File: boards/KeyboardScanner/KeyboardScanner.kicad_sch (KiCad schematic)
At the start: 20 parts, among them J1 Keyboard1, J2 Keyboard1, J3 Encoder, J4 Select, U11 TBD62783A, U8 4069

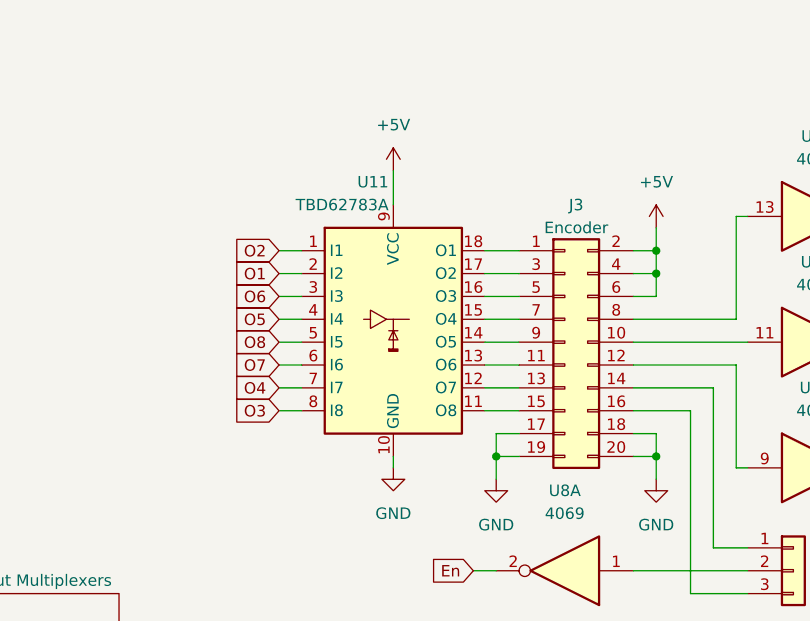
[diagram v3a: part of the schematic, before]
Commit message: Revert "Replaced inverting with non-inverting output buffer in KeyboardScanner to fix disabled open collector output"
This reverts commit 6ddf25a0a7a31b9f16f3f110cd3b7ae66d122c97.
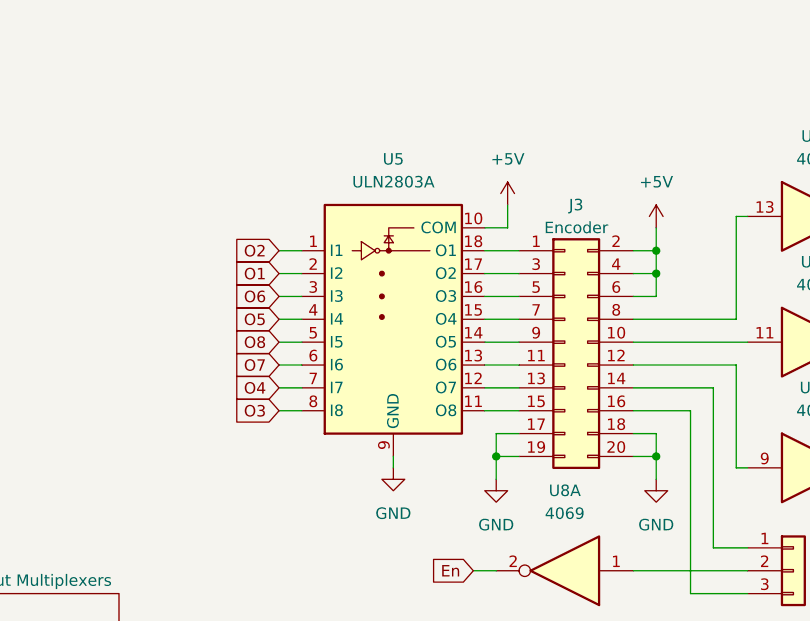
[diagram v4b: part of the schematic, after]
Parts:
- removed U11: TBD62783A, Package_DIP:DIP-18_W7.62mm, symbol Transistor_Array:TBD62783A
- added U5: ULN2803A, Package_DIP:DIP-18_W7.62mm, symbol Transistor_Array:ULN2803A
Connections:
- net +5V: now also U5.10 (COM)
- net GND: now also U5.9 (GND)
- net O1: now also U5.2 (I2)
- net O2: now also U5.1 (I1)
- net O3: now also U5.8 (I8)
- net O4: now also U5.7 (I7)
- net O5: now also U5.4 (I4)
- net O6: now also U5.3 (I3)
- net O7: now also U5.6 (I6)
- net O8: now also U5.5 (I5)
- net at J3.1 (Pin_1): now also U5.18 (O1)
- net at J3.11 (Pin_11): now also U5.13 (O6)
- net at J3.13 (Pin_13): now also U5.12 (O7)
- net at J3.15 (Pin_15): now also U5.11 (O8)
- net at J3.3 (Pin_3): now also U5.17 (O2)
- net at J3.5 (Pin_5): now also U5.16 (O3)
- net at J3.7 (Pin_7): now also U5.15 (O4)
- net at J3.9 (Pin_9): now also U5.14 (O5)
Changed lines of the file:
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@@
 	(wire
 		(pts
+			(xy 194.31 48.26) (xy 191.77 48.26)
+		)
+		(stroke
+			(width 0)
+			(type default)
+		)
+	)
+	(wire
+		(pts
 			(xy 208.28 86.36) (xy 220.98 86.36)
 		)
@@
 	(wire
 		(pts
+			(xy 194.31 45.72) (xy 194.31 48.26)
+		)
+		(stroke
+			(width 0)
+			(type default)
+		)
+	)
+	(wire
+		(pts
 			(xy 58.42 90.17) (xy 58.42 88.9)
 		)
@@
 	(wire
 		(pts
-			(xy 181.61 41.91) (xy 181.61 45.72)
-		)
-		(stroke
-			(width 0)
-			(type default)
-		)
-	)
-	(wire
-		(pts
 			(xy 45.72 76.2) (xy 63.5 76.2)
 		)
@@
 	(symbol
 		(lib_id "power:+5V")
-		(at 181.61 41.91 0)
+		(at 194.31 45.72 0)
 		(unit 1)
 		(exclude_from_sim no)
@@
 		(fields_autoplaced yes)
 		(property "Reference" "#PWR010"
-			(at 181.61 45.72 0)
+			(at 194.31 49.53 0)
 			(effects
 				(font
@@
 		)
 		(property "Value" "+5V"
-			(at 181.61 36.83 0)
+			(at 194.31 40.64 0)
 			(effects
 				(font
@@
 		)
 		(property "Footprint" ""
-			(at 181.61 41.91 0)
+			(at 194.31 45.72 0)
 			(effects
 				(font
@@
 		)
 		(property "Datasheet" ""
-			(at 181.61 41.91 0)
+			(at 194.31 45.72 0)
 			(effects
 				(font
@@
 		)
 		(property "Description" "Power symbol creates a global label with name \"+5V\""
-			(at 181.61 41.91 0)
+			(at 194.31 45.72 0)
 			(effects
 				(font
@@
 	)
 	(symbol
-		(lib_id "Transistor_Array:TBD62783A")
-		(at 181.61 58.42 0)
+		(lib_id "Device:C_Polarized")
+		(at 194.31 125.73 0)
 		(unit 1)
 		(exclude_from_sim no)
@@
 		(on_board yes)
 		(dnp no)
-		(property "Reference" "U11"
-			(at 181.0894 43.18 0)
+		(fields_autoplaced yes)
+		(property "Reference" "C10"
+			(at 198.12 123.5709 0)
 			(effects
 				(font
 					(size 1.27 1.27)
 				)
-				(justify right)
+				(justify left)
 			)
 		)
-		(property "Value" "TBD62783A"
-			(at 181.0894 45.72 0)
+		(property "Value" "47uF"
+			(at 198.12 126.1109 0)
 			(effects
 				(font
 					(size 1.27 1.27)
 				)
-				(justify right)
+				(justify left)
 			)
 		)
-		(property "Footprint" "Package_DIP:DIP-18_W7.62mm"
-			(at 181.61 72.39 0)
+		(property "Footprint" "Capacitor_THT:CP_Radial_D6.3mm_P2.50mm"
+			(at 195.2752 129.54 0)
 			(effects
 				(font
@@
 			)
 		)
-		(property "Datasheet" "http://toshiba.semicon-storage.com/info/docget.jsp?did=30523&prodName=TBD62783APG"
-			(at 173.99 48.26 0)
+		(property "Datasheet" "~"
+			(at 194.31 125.73 0)
 			(effects
 				(font
@@
 			)
 		)
-		(property "Description" "8-Channel Source Type Transistor Array, TTL and CMOS compatible, 500mA, 50V, DIP-18/SOP-18/SSOP-18/SOIC-18W"
-			(at 181.61 58.42 0)
+		(property "Description" "Polarized capacitor"
+			(at 194.31 125.73 0)
 			(effects
 				(font
@@
 			)
 		)
-		(pin "1"
-		)
-		(pin "10"
-		)
-		(pin "11"
-		)
-		(pin "12"
-		)
-		(pin "13"
-		)
-		(pin "14"
-		)
-		(pin "15"
-		)
-		(pin "16"
-		)
-		(pin "17"
-		)
-		(pin "18"
-		)
 		(pin "2"
 		)
-		(pin "3"
-		)
-		(pin "4"
-		)
-		(pin "5"
-		)
-		(pin "6"
-		)
-		(pin "7"
-		)
-		(pin "8"
-		)
-		(pin "9"
+		(pin "1"
 		)
 		(instances
 			(project "KeyboardScanner"
 				(path "/cbea9b23-a5d5-4e12-8904-2e66ea6ed837"
-					(reference "U11")
+					(reference "C10")
 					(unit 1)
 				)
@@
 	)
 	(symbol
-		(lib_id "Device:C_Polarized")
-		(at 194.31 125.73 0)
+		(lib_id "4xxx:4069")
+		(at 200.66 86.36 180)
 		(unit 1)
 		(exclude_from_sim no)
@@
 		(dnp no)
 		(fields_autoplaced yes)
-		(property "Reference" "C10"
-			(at 198.12 123.5709 0)
+		(property "Reference" "U8"
+			(at 200.66 77.47 0)
 			(effects
 				(font
 					(size 1.27 1.27)
 				)
-				(justify left)
 			)
 		)
-		(property "Value" "47uF"
-			(at 198.12 126.1109 0)
+		(property "Value" "4069"
+			(at 200.66 80.01 0)
 			(effects
 				(font
 					(size 1.27 1.27)
 				)
-				(justify left)
 			)
 		)
-		(property "Footprint" "Capacitor_THT:CP_Radial_D6.3mm_P2.50mm"
-			(at 195.2752 129.54 0)
+		(property "Footprint" "Package_DIP:DIP-14_W7.62mm"
+			(at 200.66 86.36 0)
 			(effects
 				(font
@@
 			)
 		)
-		(property "Datasheet" "~"
-			(at 194.31 125.73 0)
+		(property "Datasheet" "http://www.intersil.com/content/dam/Intersil/documents/cd40/cd4069ubms.pdf"
+			(at 200.66 86.36 0)
 			(effects
 				(font
@@
 			)
 		)
-		(property "Description" "Polarized capacitor"
-			(at 194.31 125.73 0)
+		(property "Description" "Hex inverter"
+			(at 200.66 86.36 0)
 			(effects
 				(font
@@
 			)
 		)
+		(pin "1"
+		)
 		(pin "2"
 		)
-		(pin "1"
+		(pin "3"
+		)
+		(pin "4"
+		)
+		(pin "5"
+		)
+		(pin "6"
+		)
+		(pin "8"
+		)
+		(pin "9"
+		)
+		(pin "10"
+		)
+		(pin "11"
+		)
+		(pin "12"
+		)
+		(pin "13"
+		)
+		(pin "14"
+		)
+		(pin "7"
 		)
 		(instances
 			(project "KeyboardScanner"
 				(path "/cbea9b23-a5d5-4e12-8904-2e66ea6ed837"
-					(reference "C10")
+					(reference "U8")
 					(unit 1)
 				)
@@
 	)
 	(symbol
-		(lib_id "4xxx:4069")
-		(at 200.66 86.36 180)
+		(lib_id "Transistor_Array:ULN2803A")
+		(at 181.61 55.88 0)
 		(unit 1)
 		(exclude_from_sim no)
@@
 		(dnp no)
 		(fields_autoplaced yes)
-		(property "Reference" "U8"
-			(at 200.66 77.47 0)
+		(property "Reference" "U5"
+			(at 181.61 40.64 0)
 			(effects
 				(font
@@
 			)
 		)
-		(property "Value" "4069"
-			(at 200.66 80.01 0)
+		(property "Value" "ULN2803A"
+			(at 181.61 43.18 0)
 			(effects
 				(font
@@
 			)
 		)
-		(property "Footprint" "Package_DIP:DIP-14_W7.62mm"
-			(at 200.66 86.36 0)
+		(property "Footprint" "Package_DIP:DIP-18_W7.62mm"
+			(at 182.88 72.39 0)
 			(effects
 				(font
 					(size 1.27 1.27)
 				)
+				(justify left)
 				(hide yes)
 			)
 		)
-		(property "Datasheet" "http://www.intersil.com/content/dam/Intersil/documents/cd40/cd4069ubms.pdf"
-			(at 200.66 86.36 0)
+		(property "Datasheet" "http://www.ti.com/lit/ds/symlink/uln2803a.pdf"
+			(at 184.15 60.96 0)
 			(effects
 				(font
@@
 			)
 		)
-		(property "Description" "Hex inverter"
-			(at 200.66 86.36 0)
+		(property "Description" "Darlington Transistor Arrays, SOIC18/DIP18"
+			(at 181.61 55.88 0)
 			(effects
 				(font
@@
 		(pin "1"
 		)
-		(pin "2"
+		(pin "10"
 		)
-		(pin "3"
+		(pin "11"
 		)
-		(pin "4"
+		(pin "12"
 		)
-		(pin "5"
+		(pin "13"
 		)
-		(pin "6"
+		(pin "14"
 		)
-		(pin "8"
+		(pin "15"
 		)
-		(pin "9"
+		(pin "16"
 		)
-		(pin "10"
+		(pin "17"
 		)
-		(pin "11"
+		(pin "18"
 		)
-		(pin "12"
+		(pin "2"
 		)
-		(pin "13"
+		(pin "3"
 		)
-		(pin "14"
+		(pin "4"
+		)
+		(pin "5"
+		)
+		(pin "6"
 		)
 		(pin "7"
 		)
+		(pin "8"
+		)
+		(pin "9"
+		)
 		(instances
 			(project "KeyboardScanner"
 				(path "/cbea9b23-a5d5-4e12-8904-2e66ea6ed837"
-					(reference "U8")
+					(reference "U5")
 					(unit 1)
 				)
